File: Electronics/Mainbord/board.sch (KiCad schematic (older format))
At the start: 51 parts, among them J16 Screw_Terminal_01x10, J17 Screw_Terminal_01x10, J18 Screw_Terminal_01x10, J19 Screw_Terminal_01x10, J20 Screw_Terminal_01x10, J21 Screw_Terminal_01x10, J22 Screw_Terminal_01x10, J23 Screw_Terminal_01x10, J24 Screw_Terminal_01x10, J25 Screw_Terminal_01x10, J26 Screw_Terminal_01x10, J27 Screw_Terminal_01x10, J28 Screw_Terminal_01x10, U16 PCF8575, U17 ProMicro, U18 PCF8575, U19 PCF8575, U20 74HC595, U21 74HC4051, U22 74HC4051, U23 74HC165, U24 74HC165, U25 74HC165, U26 74HC165, U27 74HC165, U28 74HC165, U29 74HC165, U30 74HC165

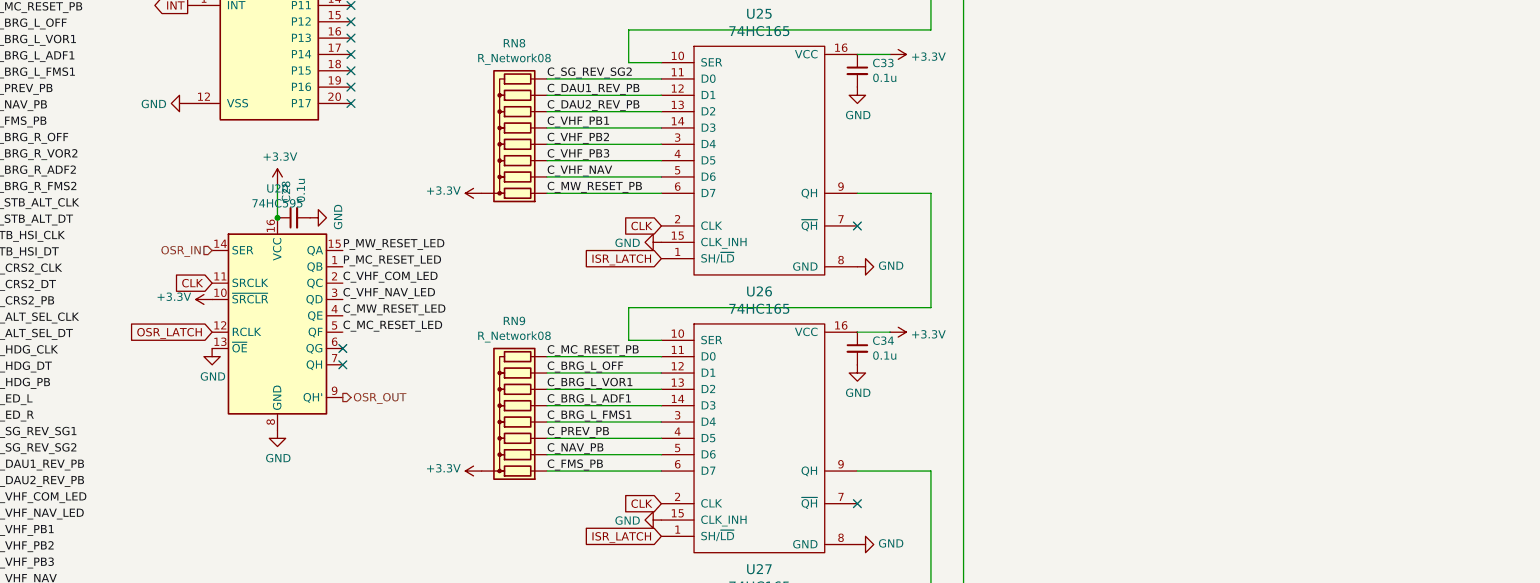
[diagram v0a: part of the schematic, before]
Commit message: Electronics - Misc works
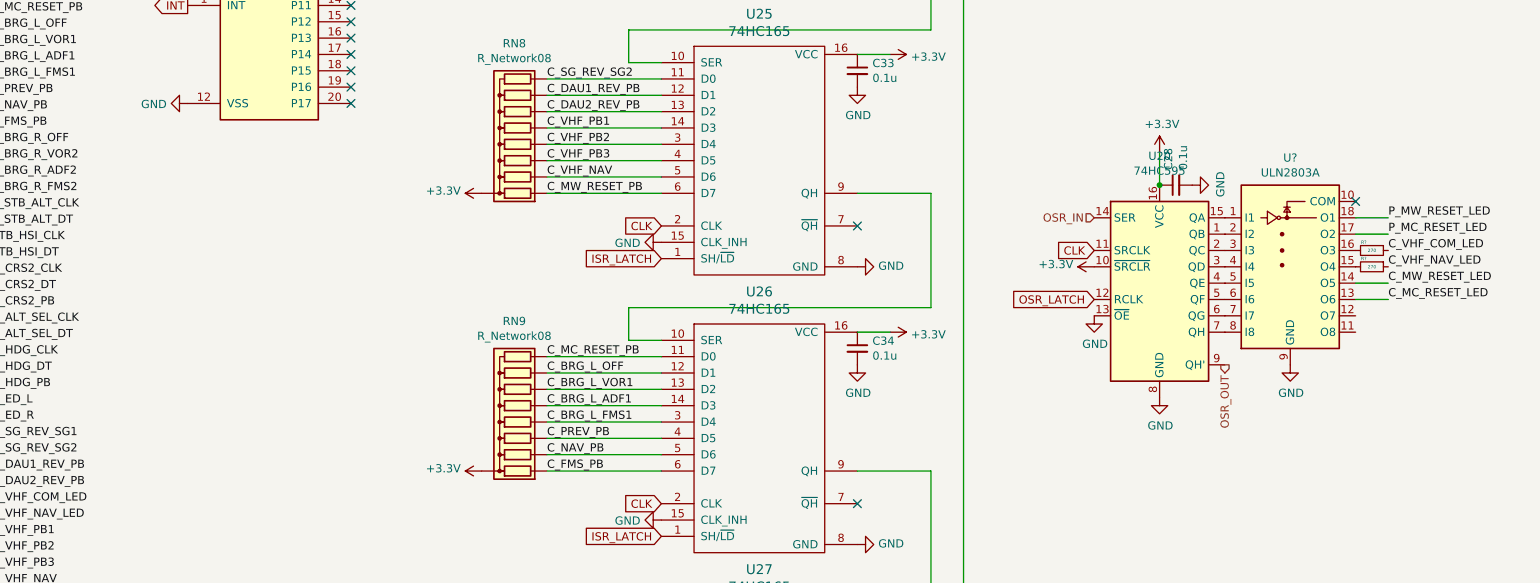
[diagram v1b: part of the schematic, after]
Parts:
- added R? (x2): 270, symbol Device:R_Small
- added U?: ULN2803A, symbol Transistor_Array:ULN2803A
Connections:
- net C_MC_RESET_LED: now also U?.13 (O6); no longer U20.5 (QF)
- net C_MW_RESET_LED: now also U?.14 (O5); no longer U20.4 (QE)
- net C_VHF_COM_LED: now also R?.1; no longer U20.2 (QC)
- net C_VHF_NAV_LED: now also R?.1; no longer U20.3 (QD)
- net GND: now also U?.9 (GND)
- net P_MC_RESET_LED: now also U?.17 (O2); no longer U20.1 (QB)
- net P_MW_RESET_LED: now also U?.18 (O1); no longer U20.15 (QA)
- net at U20.6 (QG): now also U?.7 (I7)
- net at U20.7 (QH): now also U?.8 (I8)
- new net: U20.1 (QB), U?.2 (I2)
- new net: U20.15 (QA), U?.1 (I1)
- new net: U20.2 (QC), U?.3 (I3)
- new net: U20.3 (QD), U?.4 (I4)
- new net: U20.4 (QE), U?.5 (I5)
- new net: U20.5 (QF), U?.6 (I6)
- new net: R?.2, U?.15 (O4)
- new net: R?.2, U?.16 (O3)
- no-connect marks 35 -> 34
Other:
- moved on the sheet: C28, U20
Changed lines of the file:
@@
 EESchema Schematic File Version 4
-LIBS:CitationX_cockpit-cache
-EELAYER 26 0
+EELAYER 30 0
 EELAYER END
 $Descr A3 11693 16535 portrait
 encoding utf-8
-Sheet 3 8
+Sheet 3 7
 Title ""
 Date ""
@@
 L Device:C_Small C?
 U 1 1 5DF1ADB9
-P 3600 8250
+P 9000 8050
 AR Path="/5DB5DCD1/5DF1ADB9" Ref="C?"  Part="1"
 AR Path="/5DC174D4/5DF1ADB9" Ref="C?"  Part="1"
 AR Path="/5DB6029E/5DF1ADB9" Ref="C28"  Part="1"
-F 0 "C28" H 3692 8296 50  0000 L CNN
-F 1 "0.1u" H 3692 8205 50  0000 L CNN
-F 2 "" H 3600 8250 50  0001 C CNN
-F 3 "~" H 3600 8250 50  0001 C CNN
-	1    3600 8250
+F 0 "C28" H 9092 8096 50  0000 L CNN
+F 1 "0.1u" H 9092 8005 50  0000 L CNN
+F 2 "" H 9000 8050 50  0001 C CNN
+F 3 "~" H 9000 8050 50  0001 C CNN
+	1    9000 8050
 	0    -1   -1   0
 $EndComp
@@
 L power:GND #PWR?
 U 1 1 5DF1ADC0
-P 3700 8250
+P 9100 8050
 AR Path="/5DB5DCD1/5DF1ADC0" Ref="#PWR?"  Part="1"
 AR Path="/5DC174D4/5DF1ADC0" Ref="#PWR?"  Part="1"
 AR Path="/5DB6029E/5DF1ADC0" Ref="#PWR0245"  Part="1"
-F 0 "#PWR0245" H 3700 8000 50  0001 C CNN
-F 1 "GND" H 3705 8077 50  0000 C CNN
-F 2 "" H 3700 8250 50  0001 C CNN
-F 3 "" H 3700 8250 50  0001 C CNN
-	1    3700 8250
-	0    -1   -1   0
-$EndComp
-Wire Wire Line
-	3500 8250 3500 8050
+F 0 "#PWR0245" H 9100 7800 50  0001 C CNN
+F 1 "GND" H 9105 7877 50  0000 C CNN
+F 2 "" H 9100 8050 50  0001 C CNN
+F 3 "" H 9100 8050 50  0001 C CNN
+	1    9100 8050
+	0    -1   -1   0
+$EndComp
+Wire Wire Line
+	8900 8050 8900 7850
 $Comp
 L 74xx:74HC595 U?
 U 1 1 5DF1ADC7
-P 3500 8850
+P 8900 8650
 AR Path="/5DB5DCD1/5DF1ADC7" Ref="U?"  Part="1"
 AR Path="/5DC174D4/5DF1ADC7" Ref="U?"  Part="1"
 AR Path="/5DB6029E/5DF1ADC7" Ref="U20"  Part="1"
-F 0 "U20" H 3500 9628 50  0000 C CNN
-F 1 "74HC595" H 3500 9537 50  0000 C CNN
-F 2 "" H 3500 8850 50  0001 C CNN
-F 3 "http://www.ti.com/lit/ds/symlink/sn74hc595.pdf" H 3500 8850 50  0001 C CNN
-	1    3500 8850
-	1    0    0    -1
-$EndComp
-Connection ~ 3500 8250
+F 0 "U20" H 8900 9428 50  0000 C CNN
+F 1 "74HC595" H 8900 9337 50  0000 C CNN
+F 2 "" H 8900 8650 50  0001 C CNN
+F 3 "http://www.ti.com/lit/ds/symlink/sn74hc595.pdf" H 8900 8650 50  0001 C CNN
+	1    8900 8650
+	1    0    0    -1
+$EndComp
+Connection ~ 8900 8050
 $Comp
 L power:GND #PWR?
 U 1 1 5DF1ADCF
-P 3500 9550
+P 8900 9350
 AR Path="/5DB5DCD1/5DF1ADCF" Ref="#PWR?"  Part="1"
 AR Path="/5DC174D4/5DF1ADCF" Ref="#PWR?"  Part="1"
 AR Path="/5DB6029E/5DF1ADCF" Ref="#PWR0246"  Part="1"
-F 0 "#PWR0246" H 3500 9300 50  0001 C CNN
-F 1 "GND" H 3505 9377 50  0000 C CNN
-F 2 "" H 3500 9550 50  0001 C CNN
-F 3 "" H 3500 9550 50  0001 C CNN
-	1    3500 9550
-	1    0    0    -1
-$EndComp
-Text HLabel 3100 8450 0    50   Input ~ 0
+F 0 "#PWR0246" H 8900 9100 50  0001 C CNN
+F 1 "GND" H 8905 9177 50  0000 C CNN
+F 2 "" H 8900 9350 50  0001 C CNN
+F 3 "" H 8900 9350 50  0001 C CNN
+	1    8900 9350
+	1    0    0    -1
+$EndComp
+Text HLabel 8500 8250 0    50   Input ~ 0
 OSR_IN
 $Comp
 L power:GND #PWR?
 U 1 1 5DF1ADD6
-P 3100 9050
+P 8500 8850
 AR Path="/5DB5DCD1/5DF1ADD6" Ref="#PWR?"  Part="1"
 AR Path="/5DC174D4/5DF1ADD6" Ref="#PWR?"  Part="1"
 AR Path="/5DB6029E/5DF1ADD6" Ref="#PWR0247"  Part="1"
-F 0 "#PWR0247" H 3100 8800 50  0001 C CNN
-F 1 "GND" H 3105 8877 50  0000 C CNN
-F 2 "" H 3100 9050 50  0001 C CNN
-F 3 "" H 3100 9050 50  0001 C CNN
-	1    3100 9050
+F 0 "#PWR0247" H 8500 8600 50  0001 C CNN
+F 1 "GND" H 8505 8677 50  0000 C CNN
+F 2 "" H 8500 8850 50  0001 C CNN
+F 3 "" H 8500 8850 50  0001 C CNN
+	1    8500 8850
 	1    0    0    -1
 $EndComp
@@
 L power:+3.3V #PWR?
 U 1 1 5DF1ADDD
-P 3500 8050
+P 8900 7850
 AR Path="/5DB5DCD1/5DF1ADDD" Ref="#PWR?"  Part="1"
 AR Path="/5DC174D4/5DF1ADDD" Ref="#PWR?"  Part="1"
 AR Path="/5DB6029E/5DF1ADDD" Ref="#PWR0248"  Part="1"
-F 0 "#PWR0248" H 3500 7900 50  0001 C CNN
-F 1 "+3.3V" H 3515 8223 50  0000 C CNN
-F 2 "" H 3500 8050 50  0001 C CNN
-F 3 "" H 3500 8050 50  0001 C CNN
-	1    3500 8050
+F 0 "#PWR0248" H 8900 7700 50  0001 C CNN
+F 1 "+3.3V" H 8915 8023 50  0000 C CNN
+F 2 "" H 8900 7850 50  0001 C CNN
+F 3 "" H 8900 7850 50  0001 C CNN
+	1    8900 7850
 	1    0    0    -1
 $EndComp
@@
 L power:+3.3V #PWR?
 U 1 1 5DF1ADE3
-P 3100 8750
+P 8500 8550
 AR Path="/5DB5DCD1/5DF1ADE3" Ref="#PWR?"  Part="1"
 AR Path="/5DC174D4/5DF1ADE3" Ref="#PWR?"  Part="1"
 AR Path="/5DB6029E/5DF1ADE3" Ref="#PWR0249"  Part="1"
-F 0 "#PWR0249" H 3100 8600 50  0001 C CNN
-F 1 "+3.3V" V 3115 8878 50  0000 L CNN
-F 2 "" H 3100 8750 50  0001 C CNN
-F 3 "" H 3100 8750 50  0001 C CNN
-	1    3100 8750
-	0    -1   -1   0
-$EndComp
-Text GLabel 3100 8650 0    50   Input ~ 0
+F 0 "#PWR0249" H 8500 8400 50  0001 C CNN
+F 1 "+3.3V" V 8515 8678 50  0000 L CNN
+F 2 "" H 8500 8550 50  0001 C CNN
+F 3 "" H 8500 8550 50  0001 C CNN
+	1    8500 8550
+	0    -1   -1   0
+$EndComp
+Text GLabel 8500 8450 0    50   Input ~ 0
 CLK
-Text Label 3900 8450 0    50   ~ 0
-P_MW_RESET_LED
 Text Label 5150 4000 0    50   ~ 0
 P_MW_RESET_PB
-Text Label 3900 8550 0    50   ~ 0
-P_MC_RESET_LED
 Text Label 5150 4100 0    50   ~ 0
 P_MC_RESET_PB
@@
 Text Label 4000 4550 0    50   ~ 0
 C_VHF_PB
-Text Label 3900 8850 0    50   ~ 0
-C_MW_RESET_LED
 Text Label 5150 8100 0    50   ~ 0
 C_MW_RESET_PB
-Text Label 3900 8950 0    50   ~ 0
-C_MC_RESET_LED
 Text Label 5150 9100 0    50   ~ 0
 C_MC_RESET_PB
@@
 Text Label 4000 4750 0    50   ~ 0
 P_MIN_DT
-Text Label 3900 8650 0    50   ~ 0
-C_VHF_COM_LED
-Text Label 3900 8750 0    50   ~ 0
-C_VHF_NAV_LED
 Text Label 1750 12700 0    50   ~ 0
 P_STD_PB
@@
 Text Label 1750 15900 0    50   ~ 0
 C_BARO_DT
-Text HLabel 3900 9350 2    50   Output ~ 0
+Text HLabel 9300 9150 3    50   Output ~ 0
 OSR_OUT
 $Comp
@@
 Wire Wire Line
 	5150 11000 5850 11000
-NoConn ~ 3900 9050
-NoConn ~ 3900 9150
 NoConn ~ 1950 5500
 NoConn ~ 3950 6650
@@
 Text GLabel 2950 6950 0    50   Output ~ 0
 INT
-Text GLabel 3100 8950 0    50   Input ~ 0
+Text GLabel 8500 8750 0    50   Input ~ 0
 OSR_LATCH
+$Comp
+L Transistor_Array:ULN2803A U?
+U 1 1 5DF8E5E4
+P 9700 8450
+F 0 "U?" H 9700 9017 50  0000 C CNN
+F 1 "ULN2803A" H 9700 8926 50  0000 C CNN
+F 2 "" H 9750 7800 50  0001 L CNN
+F 3 "http://www.ti.com/lit/ds/symlink/uln2803a.pdf" H 9800 8250 50  0001 C CNN
+	1    9700 8450
+	1    0    0    -1
+$EndComp
+$Comp
+L power:GND #PWR?
+U 1 1 5DF90A33
+P 9700 9150
+AR Path="/5DB5DCD1/5DF90A33" Ref="#PWR?"  Part="1"
+AR Path="/5DC174D4/5DF90A33" Ref="#PWR?"  Part="1"
+AR Path="/5DB6029E/5DF90A33" Ref="#PWR?"  Part="1"
+F 0 "#PWR?" H 9700 8900 50  0001 C CNN
+F 1 "GND" H 9705 8977 50  0000 C CNN
+F 2 "" H 9700 9150 50  0001 C CNN
+F 3 "" H 9700 9150 50  0001 C CNN
+	1    9700 9150
+	1    0    0    -1
+$EndComp
+$Comp
+L Device:R_Small R?
+U 1 1 5DFBCA65
+P 10200 8450
+AR Path="/5DC33C09/5DFBCA65" Ref="R?"  Part="1"
+AR Path="/5DB6029E/5DFBCA65" Ref="R?"  Part="1"
+F 0 "R?" V 10150 8400 20  0000 C CNN
+F 1 "270" V 10200 8450 20  0000 C CNN
+F 2 "" H 10200 8450 50  0001 C CNN
+F 3 "~" H 10200 8450 50  0001 C CNN
+	1    10200 8450
+	0    1    1    0
+$EndComp
+Text Label 10300 8550 0    50   ~ 0
+C_VHF_NAV_LED
+Text Label 10300 8450 0    50   ~ 0
+C_VHF_COM_LED
+Text Label 10300 8750 0    50   ~ 0
+C_MC_RESET_LED
+Text Label 10300 8650 0    50   ~ 0
+C_MW_RESET_LED
+Text Label 10300 8350 0    50   ~ 0
+P_MC_RESET_LED
+Text Label 10300 8250 0    50   ~ 0
+P_MW_RESET_LED
+$Comp
+L Device:R_Small R?
+U 1 1 5DFE47EA
+P 10200 8550
+AR Path="/5DC33C09/5DFE47EA" Ref="R?"  Part="1"
+AR Path="/5DB6029E/5DFE47EA" Ref="R?"  Part="1"
+F 0 "R?" V 10150 8500 20  0000 C CNN
+F 1 "270" V 10200 8550 20  0000 C CNN
+F 2 "" H 10200 8550 50  0001 C CNN
+F 3 "~" H 10200 8550 50  0001 C CNN
+	1    10200 8550
+	0    1    1    0
+$EndComp
+Wire Wire Line
+	10100 8650 10300 8650
+Wire Wire Line
+	10300 8750 10100 8750
+Wire Wire Line
+	10100 8350 10300 8350
+Wire Wire Line
+	10300 8250 10100 8250
+NoConn ~ 10100 8150
 $EndSCHEMATC
